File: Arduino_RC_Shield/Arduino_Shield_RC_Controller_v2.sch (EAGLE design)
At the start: 10 parts, among them SW1 PTS810SJG250SMTRLFS, SW2 PTS810SJG250SMTRLFS, SW3 PTS810SJG250SMTRLFS

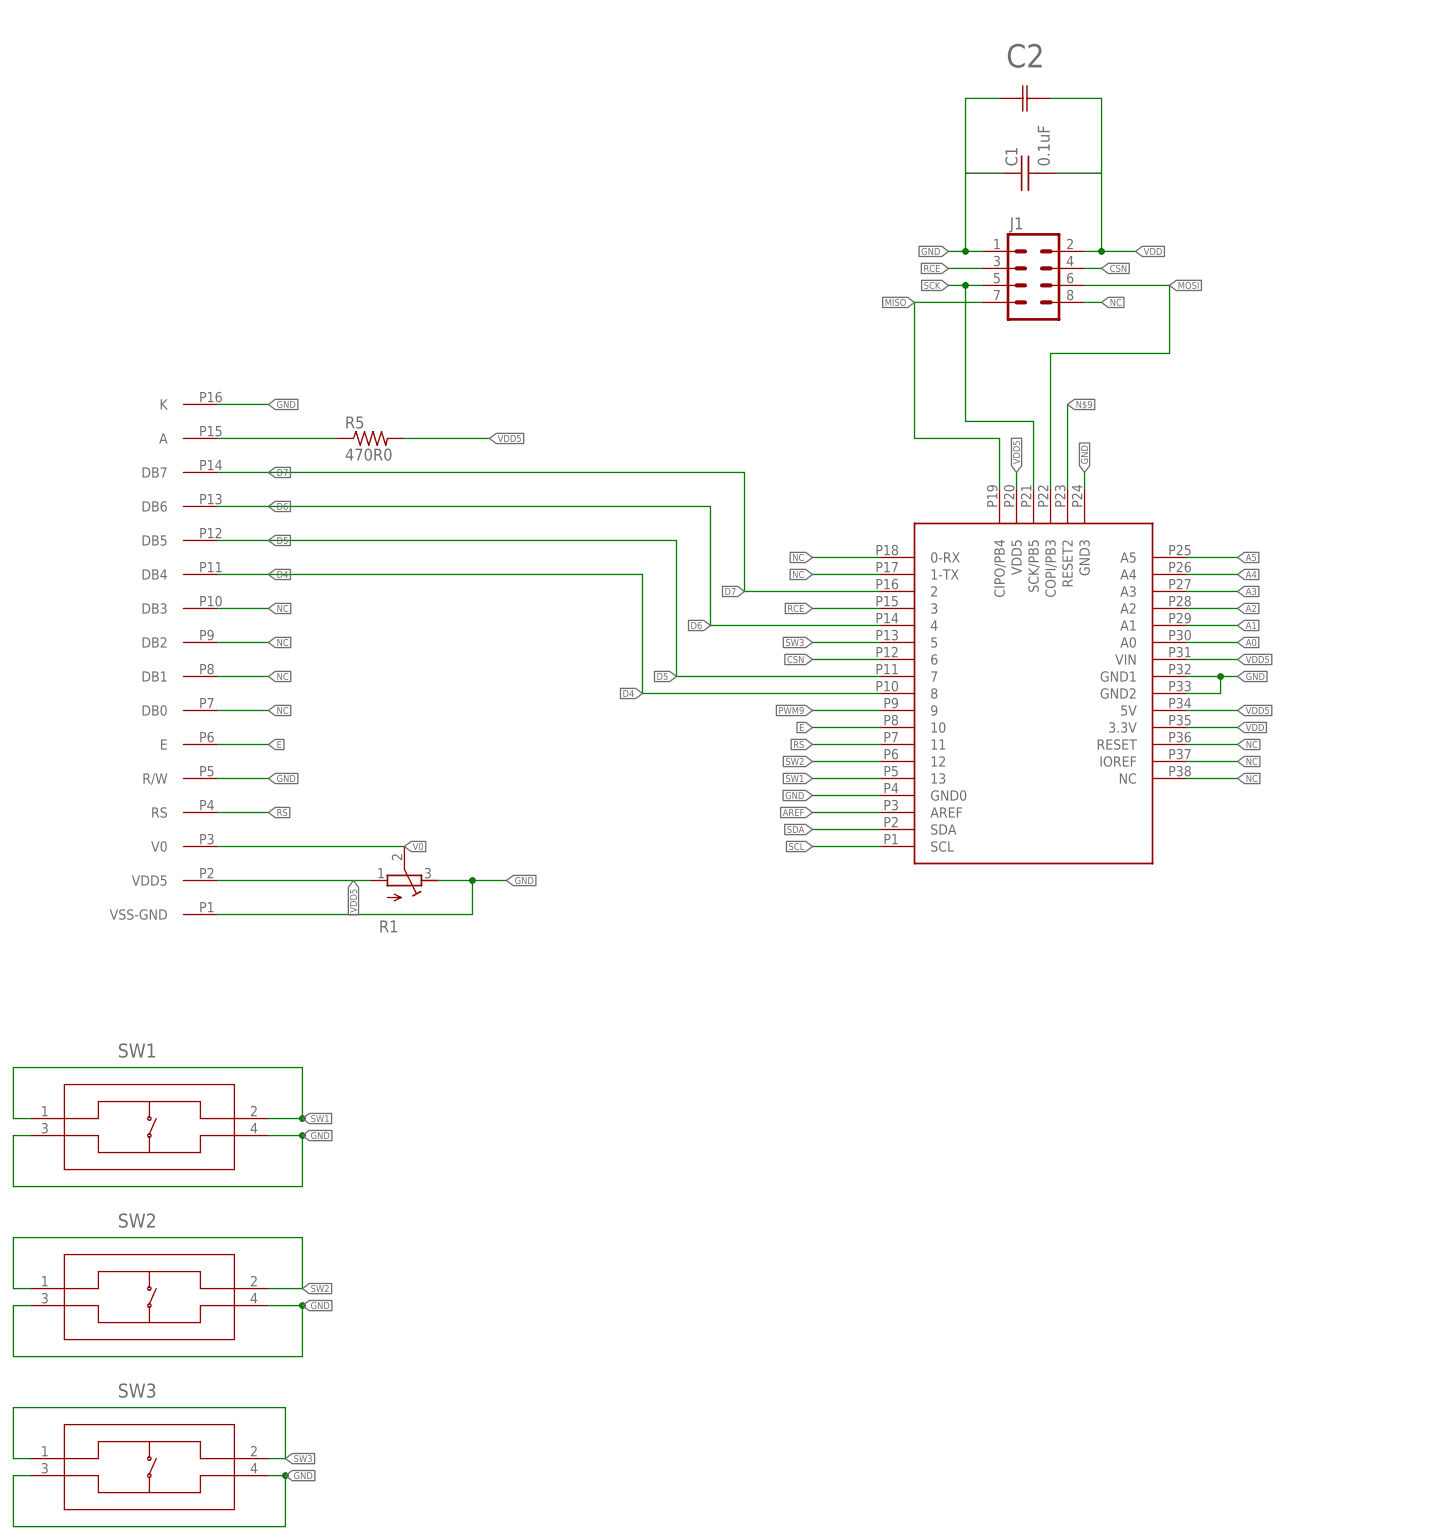
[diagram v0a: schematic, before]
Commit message: updated
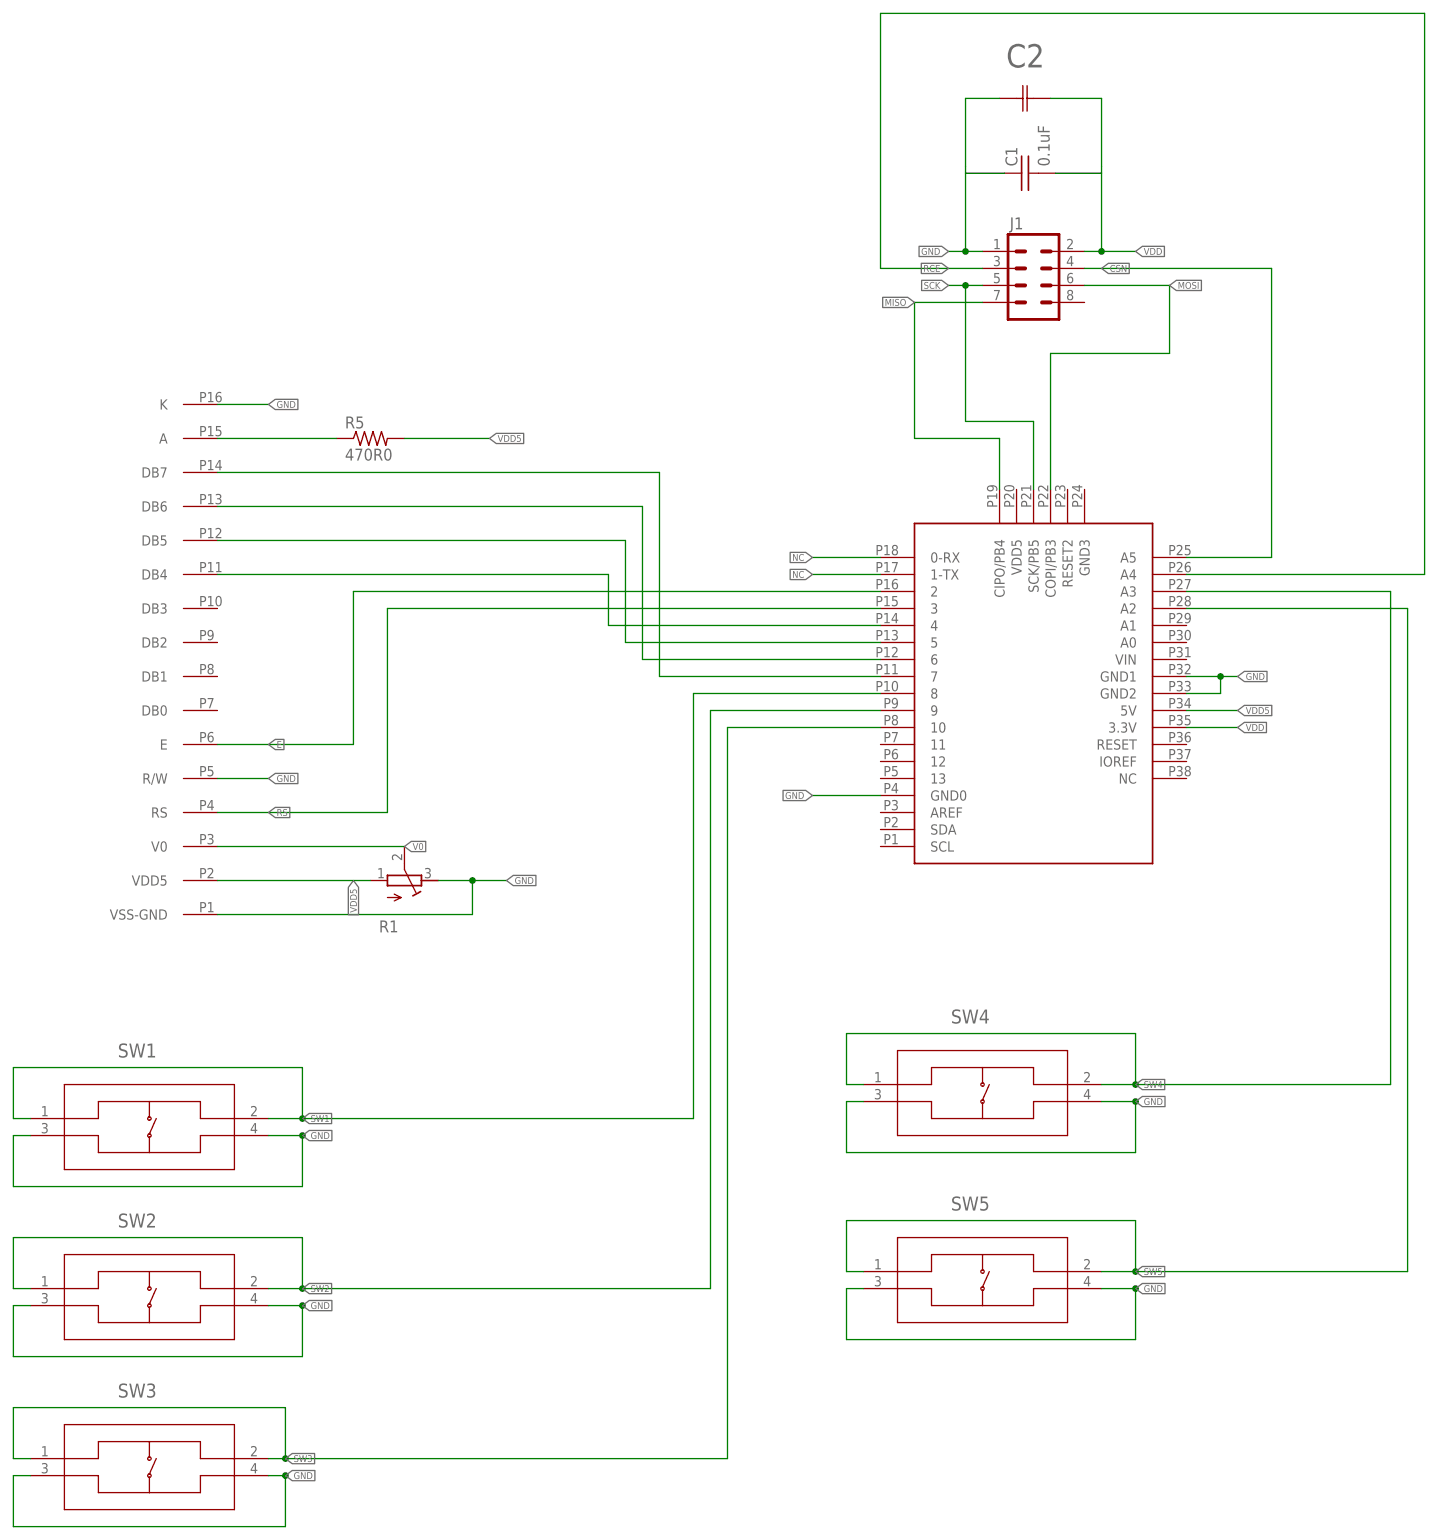
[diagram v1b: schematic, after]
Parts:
- added SW4, SW5: PTS810SJG250SMTRLFS, 3D_MIG_Controller:PTS810SJG250SMTRLFS
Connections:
- removed net A0: AR1.A0
- removed net A1: AR1.A1
- removed net A2: AR1.A2
- removed net A3: AR1.A3
- removed net A4: AR1.A4
- removed net A5: AR1.A5
- removed net AREF: AR1.AREF
- removed net D4: AR1.8, LCD1.DB4
- removed net D5: AR1.7, LCD1.DB5
- removed net D6: AR1.4, LCD1.DB6
- removed net D7: AR1.2, LCD1.DB7
- removed net N$9: AR1.RESET2
- removed net PWM9: AR1.9
- removed net SCL: AR1.SCL
- removed net SDA: AR1.SDA
- new net N$3: AR1.7, LCD1.DB7
- new net N$4: AR1.6, LCD1.DB6
- new net N$5: AR1.5, LCD1.DB5
- new net N$6: AR1.4, LCD1.DB4
- new net SW4: AR1.A3, SW4.1, SW4.2
- new net SW5: AR1.A2, SW5.1, SW5.2
- net CSN: now also AR1.A5; no longer AR1.6
- net E: now also AR1.2; no longer AR1.10
- net GND: now also SW4.3, SW4.4, SW5.3, SW5.4; no longer AR1.GND3
- net NC: no longer AR1.IOREF, AR1.NC, AR1.RESET, J1.8, LCD1.DB0, LCD1.DB1, LCD1.DB2, LCD1.DB3
- net RCE: now also AR1.A4; no longer AR1.3
- net RS: now also AR1.3; no longer AR1.11
- net SW1: now also AR1.8; no longer AR1.13
- net SW2: now also AR1.9; no longer AR1.12
- net SW3: now also AR1.10; no longer AR1.5
- net VDD5: no longer AR1.VDD5, AR1.VIN
